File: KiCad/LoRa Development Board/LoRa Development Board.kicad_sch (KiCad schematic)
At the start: 1 part

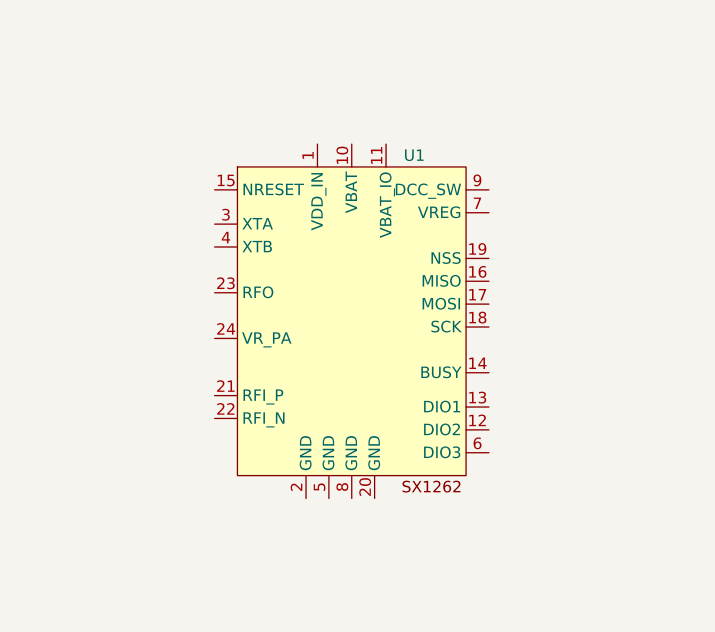
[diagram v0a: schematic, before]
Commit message: Update LoRa Board Schematic
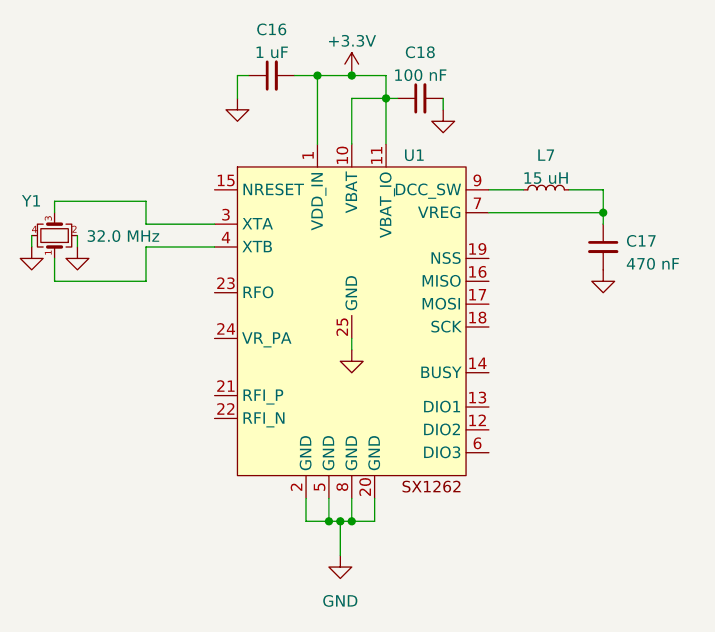
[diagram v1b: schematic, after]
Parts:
- added C16: 1 uF, symbol Device:C_Small
- added C17: 470 nF, symbol Device:C_Small
- added C18: 100 nF, symbol Device:C_Small
- added L7: 15 uH, symbol Device:L_Small
- added Y1: 32.0 MHz, symbol Device:Crystal_GND24_Small
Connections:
- net +3.3V: now reaches U1.1 (VDD_IN)
- net +3.3V: now also U1.10 (VBAT), U1.11 (VBAT_IO), C16.2, C18.1
- net GND: now reaches U1.2 (GND)
- net GND: now also U1.20 (GND), U1.25 (GND), U1.5 (GND), U1.8 (GND), C16.1, C17.2, C18.2, Y1.2, Y1.4
- net at U1.3 (XTA): now also Y1.3
- net at U1.4 (XTB): now also Y1.1
- net at U1.7 (VREG): now also C17.1, L7.2
- net at U1.9 (DCC_SW): now also L7.1
